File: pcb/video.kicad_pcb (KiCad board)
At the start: 4 copper layers, 159.9 x 99.9 mm, 174 parts, among them J1 09031966921, J3 Conn_01x06, J4 Conn_01x06, J5 Conn_01x06, J6 Conn_01x06, J7 DB15_Female_HighDensity, J8 HDMI_A, U1 NCP115, U10 NCA9306DPH, U2 LP3853ESX-3.3/NOPB, U3 LCMXO2-1200HC-4TG100I, U4 LCMXO2-7000HC-4TG144C, U5 THS8136, U6 TFP410PAP, U7 ESD224DQA, U8 ESD224DQA, U9 PCA9540BDP, X1 ASV-xxxMHz

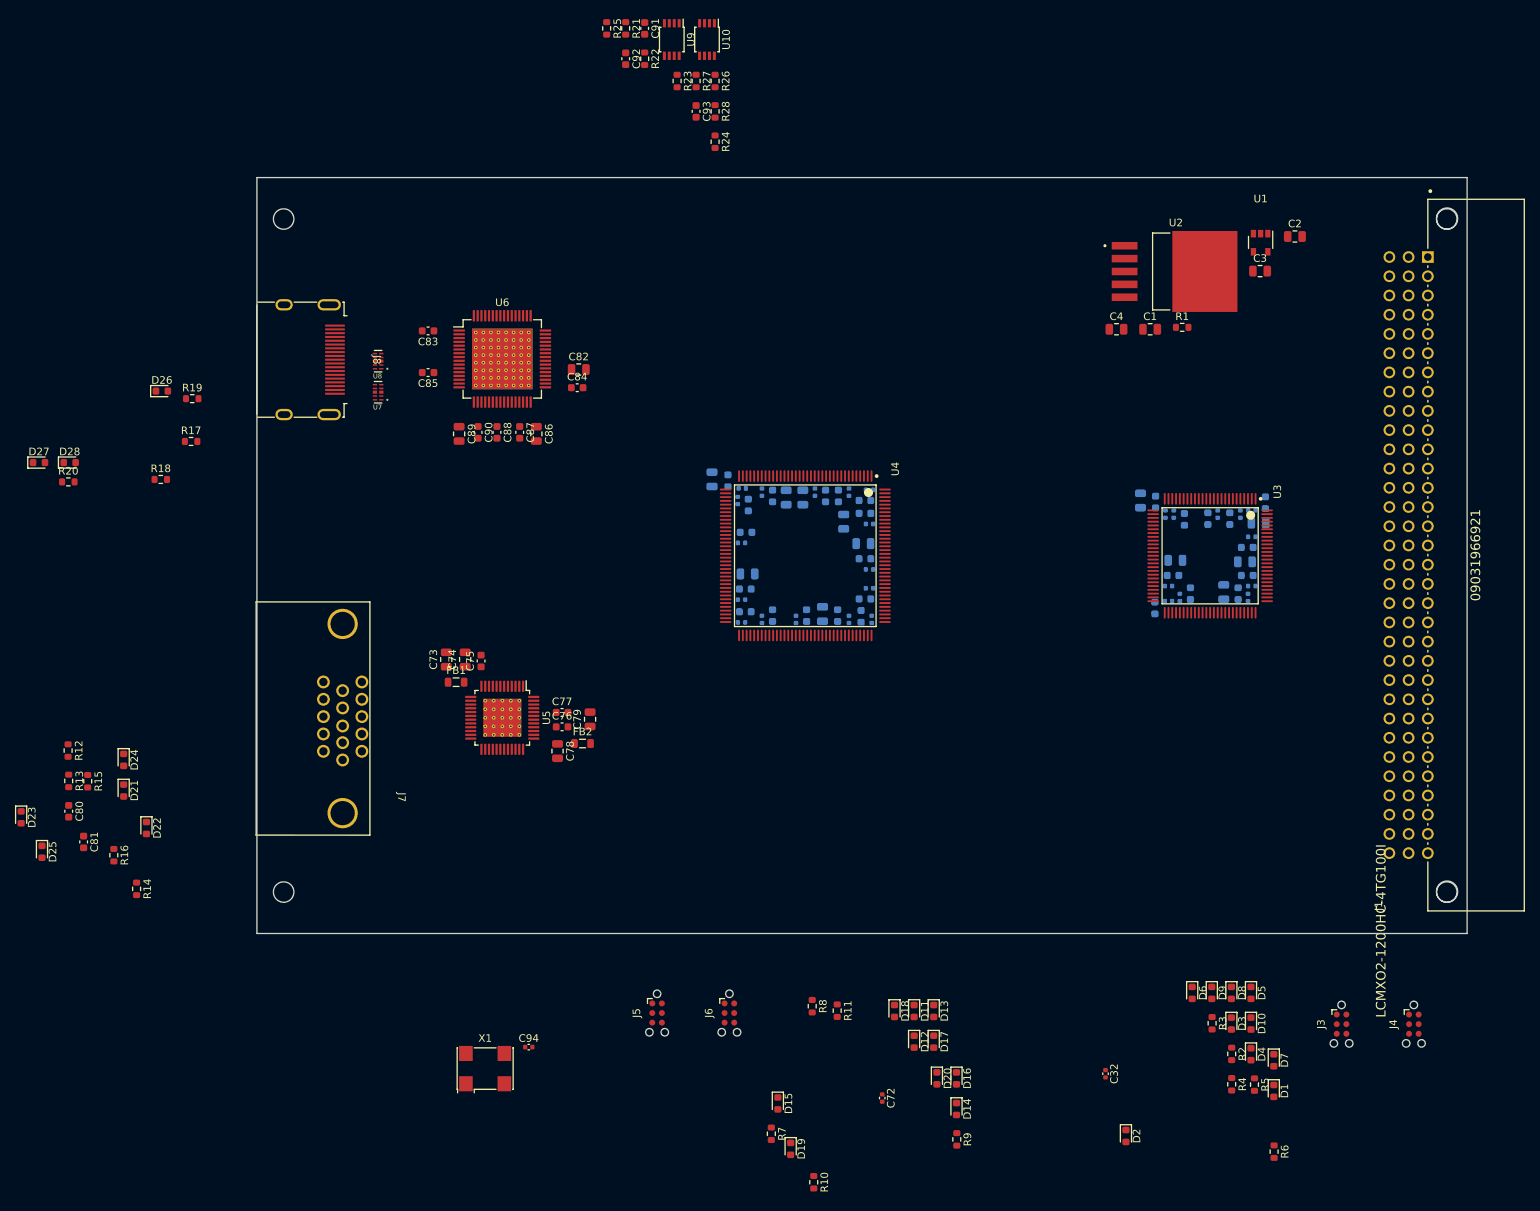
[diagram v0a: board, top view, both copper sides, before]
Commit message: place components around connectors
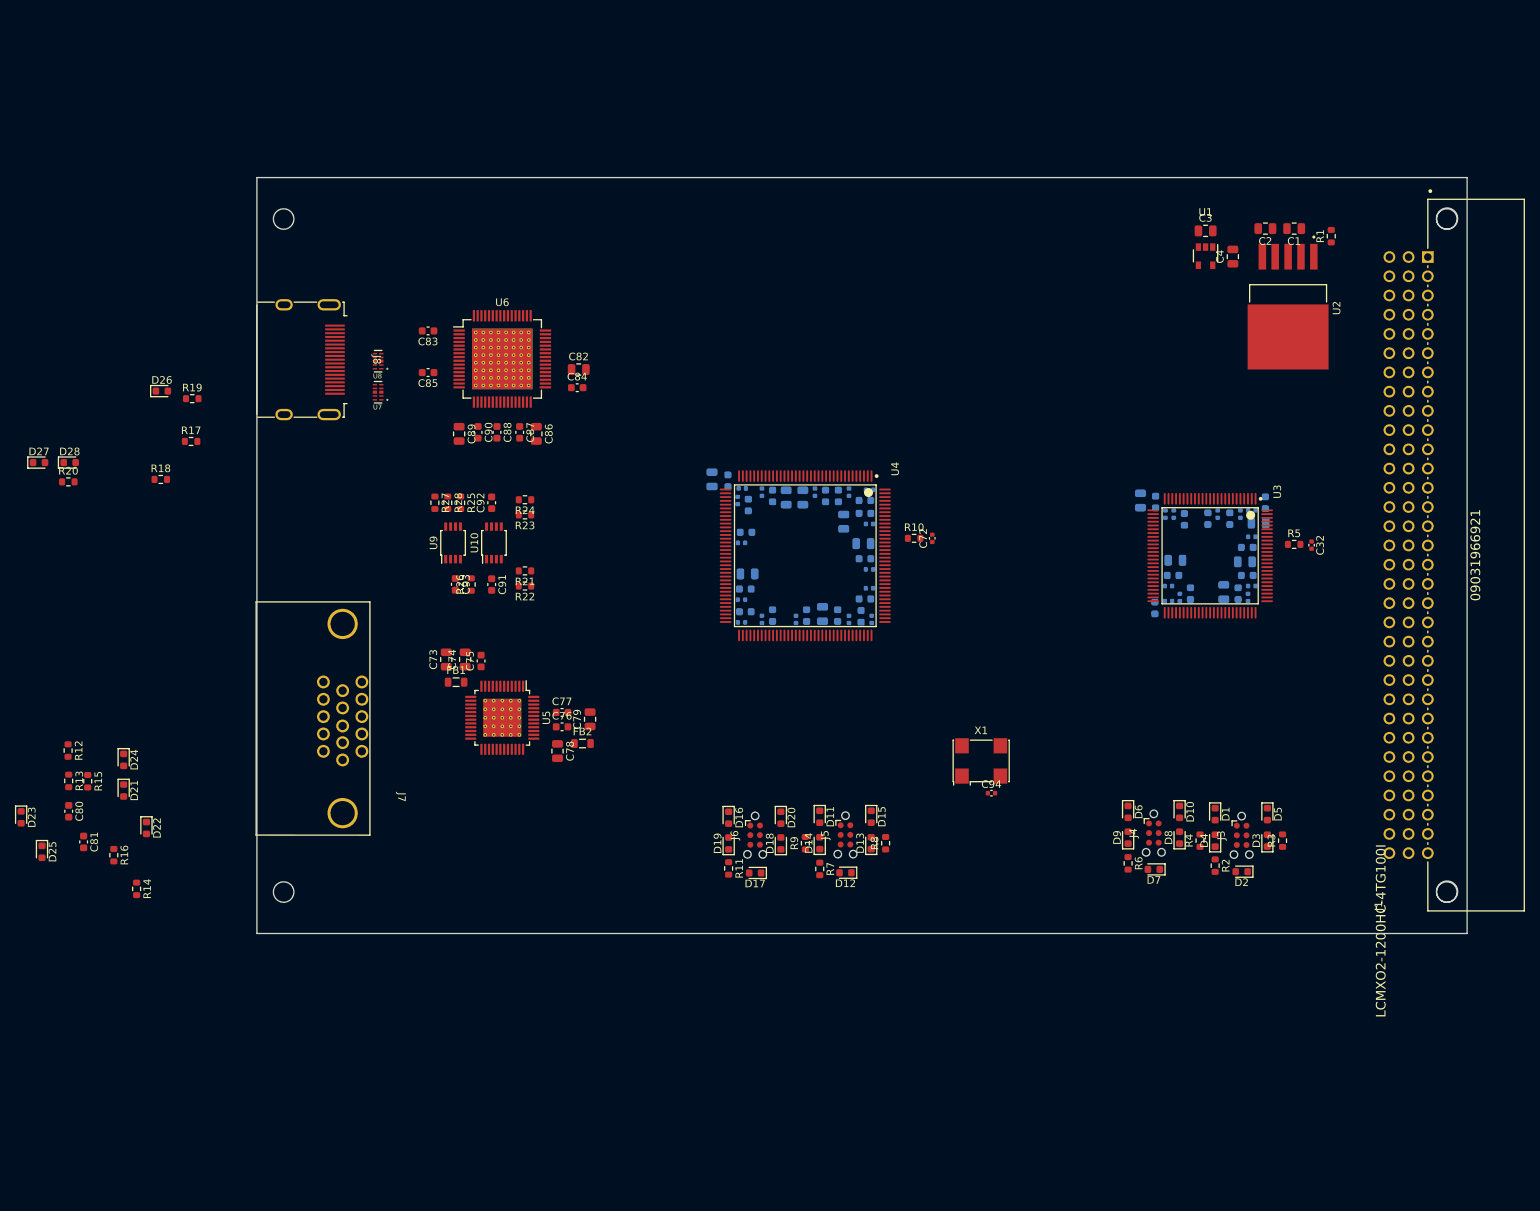
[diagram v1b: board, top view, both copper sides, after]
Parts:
- moved R10 86.1 mm to (141.9, 92.7), turned to 0 degrees
- moved X1 77.1 mm to (150.7, 122.1)
- moved C91 76.2 mm to (86.1, 98.8)
- moved C32 74.9 mm to (194.4, 93.6)
- moved C72 74.2 mm to (144.3, 92.7), turned to 90 degrees
- moved R26 73.9 mm to (83.4, 98.8), turned to 90 degrees
- moved R21 72.9 mm to (90.5, 97.0), turned to 180 degrees
- moved U9 72.5 mm to (81.0, 93.3), turned to 90 degrees
- moved U10 72.2 mm to (86.4, 93.3), turned to 90 degrees
- moved R5 71.5 mm to (192.1, 93.5), turned to 0 degrees
- moved R22 71.4 mm to (90.5, 99.0), turned to 180 degrees
- moved C93 70.1 mm to (81.3, 98.8)
- moved C94 69.7 mm to (152.1, 126.4)
- moved R25 65.6 mm to (82.0, 88.0)
- moved R27 65.5 mm to (78.6, 88.0)
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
